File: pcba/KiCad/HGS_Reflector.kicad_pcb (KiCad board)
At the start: 4 copper layers, 100 x 100 mm, 62 parts, among them J1 U.FL, J2 USB_C_Plug_USB2.0, J3 SM06B-SRSS-TB(LF)(SN), J5 132134-10, J7 USB_HOST_W/CHASSIS_GND, U1 LP2985-N, U2 TQP3M9037, U4 QPQ1907, U5 LP2985-N, U7 TQP3M9037, U8 B39162B9417K610

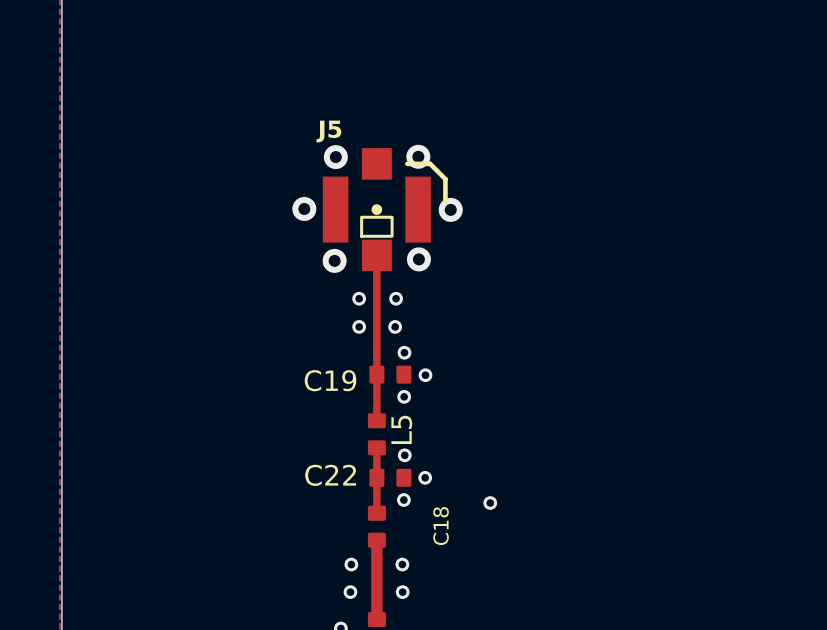
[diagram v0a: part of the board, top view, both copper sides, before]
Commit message: minor layout changes
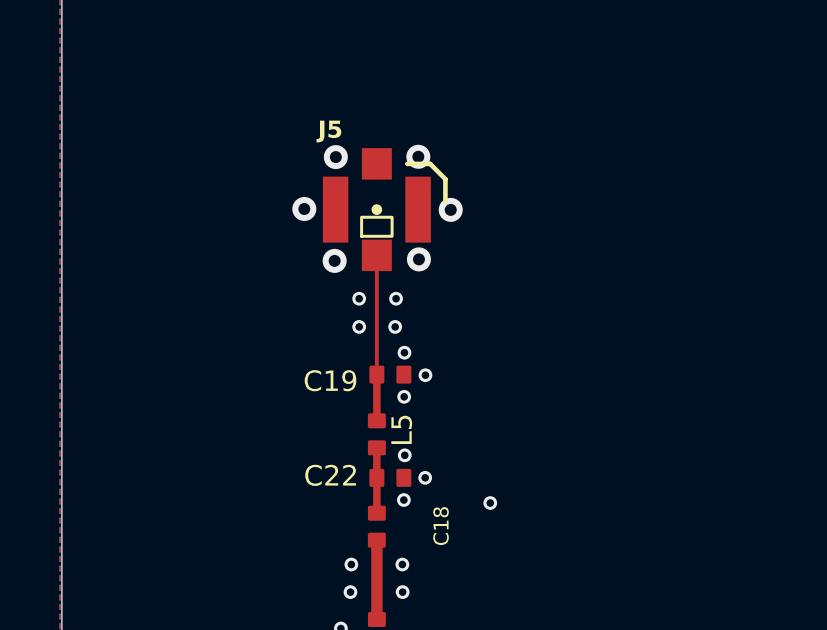
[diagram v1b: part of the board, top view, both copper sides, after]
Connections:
- net Net-(C18-Pad2) renamed /RF2
- net Net-(J5-SIGNAL) renamed /RF1
- net Net-(U2-RF_IN) renamed /RF3
- net Net-(U2-RF_OUT) renamed /RF4
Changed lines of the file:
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@@
 	(net 7 "VBUS")
 	(net 8 "Net-(C18-Pad1)")
-	(net 9 "Net-(U2-RF_IN)")
+	(net 9 "/RF3")
 	(net 10 "Net-(U1-BYPASS)")
 	(net 11 "Net-(U1-VOUT)")
@@
 	(net 13 "Net-(C11-Pad1)")
 	(net 14 "Net-(U4-IN)")
-	(net 15 "Net-(U2-RF_OUT)")
+	(net 15 "/RF4")
 	(net 16 "Net-(U5-BYPASS)")
 	(net 17 "Net-(U5-VOUT)")
@@
 	(net 25 "Net-(E5-Pad1)")
 	(net 26 "Net-(J1-SIGNAL)")
-	(net 27 "Net-(C18-Pad2)")
+	(net 27 "/RF2")
 	(net 28 "Net-(J7-D-)")
 	(net 29 "Net-(J3-Pad6)")
@@
 	(net 44 "unconnected-(J2-D+-PadA6)")
 	(net 45 "unconnected-(J2-D--PadA7)")
-	(net 46 "Net-(J5-SIGNAL)")
+	(net 46 "/RF1")
 	(net 47 "Net-(D1-A)")
 	(net 48 "Net-(D2-A)")
@@
 			(layers "F.Cu" "F.Paste")
 			(roundrect_rratio 0.1)
-			(net 15 "Net-(U2-RF_OUT)")
+			(net 15 "/RF4")
 			(pintype "passive")
 			(solder_mask_margin 0.1016)
@@
 			(layers "F.Cu" "F.Paste")
 			(roundrect_rratio 0.1)
-			(net 46 "Net-(J5-SIGNAL)")
+			(net 46 "/RF1")
 			(pintype "passive")
 			(solder_mask_margin 0.1016)
@@
 			(layers "F.Cu" "F.Paste")
 			(roundrect_rratio 0.1)
-			(net 27 "Net-(C18-Pad2)")
+			(net 27 "/RF2")
 			(pintype "passive")
 			(solder_mask_margin 0.1016)
@@
 			(layers "F.Cu" "F.Paste")
 			(roundrect_rratio 0.1)
-			(net 46 "Net-(J5-SIGNAL)")
+			(net 46 "/RF1")
 			(pinfunction "1")
 			(pintype "passive")
@@
 			(layers "F.Cu" "F.Paste")
 			(roundrect_rratio 0.1)
-			(net 27 "Net-(C18-Pad2)")
+			(net 27 "/RF2")
 			(pinfunction "2")
 			(pintype "passive")
@@
 			(layers "F.Cu" "F.Paste")
 			(roundrect_rratio 0.1)
-			(net 27 "Net-(C18-Pad2)")
+			(net 27 "/RF2")
 			(pintype "passive")
 			(solder_mask_margin 0.1016)
@@
 			(size 1.05 1)
 			(layers "F.Cu" "F.Paste" "F.Mask")
-			(net 46 "Net-(J5-SIGNAL)")
+			(net 46 "/RF1")
 			(pinfunction "SIGNAL")
 			(pintype "bidirectional")
@@
 			(size 1.2 1.6)
 			(layers "F.Cu" "F.Paste" "F.Mask")
-			(net 15 "Net-(U2-RF_OUT)")
+			(net 15 "/RF4")
 			(pintype "passive")
 			(solder_mask_margin 0.0635)
@@
 			(size 0.3 0.75)
 			(layers "F.Cu" "F.Paste" "F.Mask")
-			(net 9 "Net-(U2-RF_IN)")
+			(net 9 "/RF3")
 			(pinfunction "RF_IN")
 			(pintype "passive")
@@
 			(size 0.3 0.75)
 			(layers "F.Cu" "F.Paste" "F.Mask")
-			(net 15 "Net-(U2-RF_OUT)")
+			(net 15 "/RF4")
 			(pinfunction "RF_OUT")
 			(pintype "passive")
@@
 			(layers "F.Cu" "F.Paste")
 			(roundrect_rratio 0.1)
-			(net 9 "Net-(U2-RF_IN)")
+			(net 9 "/RF3")
 			(pintype "passive")
 			(solder_mask_margin 0.1016)
@@
 		(start 108.9989 83.5389)
 		(end 109 83.54)
-		(width 0.25)
+		(width 0.127)
 		(layer "F.Cu")
 		(net 46)
@@
 		(start 108.9989 79.565)
 		(end 108.9989 83.5389)
-		(width 0.25)
+		(width 0.127)
 		(layer "F.Cu")
 		(net 46)
